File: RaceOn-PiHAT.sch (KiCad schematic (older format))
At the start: 66 parts, among them IC1 MIC29302WU, IC2 NCP5901B, IC3 NCP5901B, IC4 BD48K60G, IC5 LMR14030, J1 BATTERY, J2 ACCELEROMETER, J3 Pi Connector, J4 Encoder Left, J5 Encoder Right, M1 SERVO, M2 MOTOR, Q1 Si7288DP, Q2 Si7288DP, Q3 SQJA37EP1

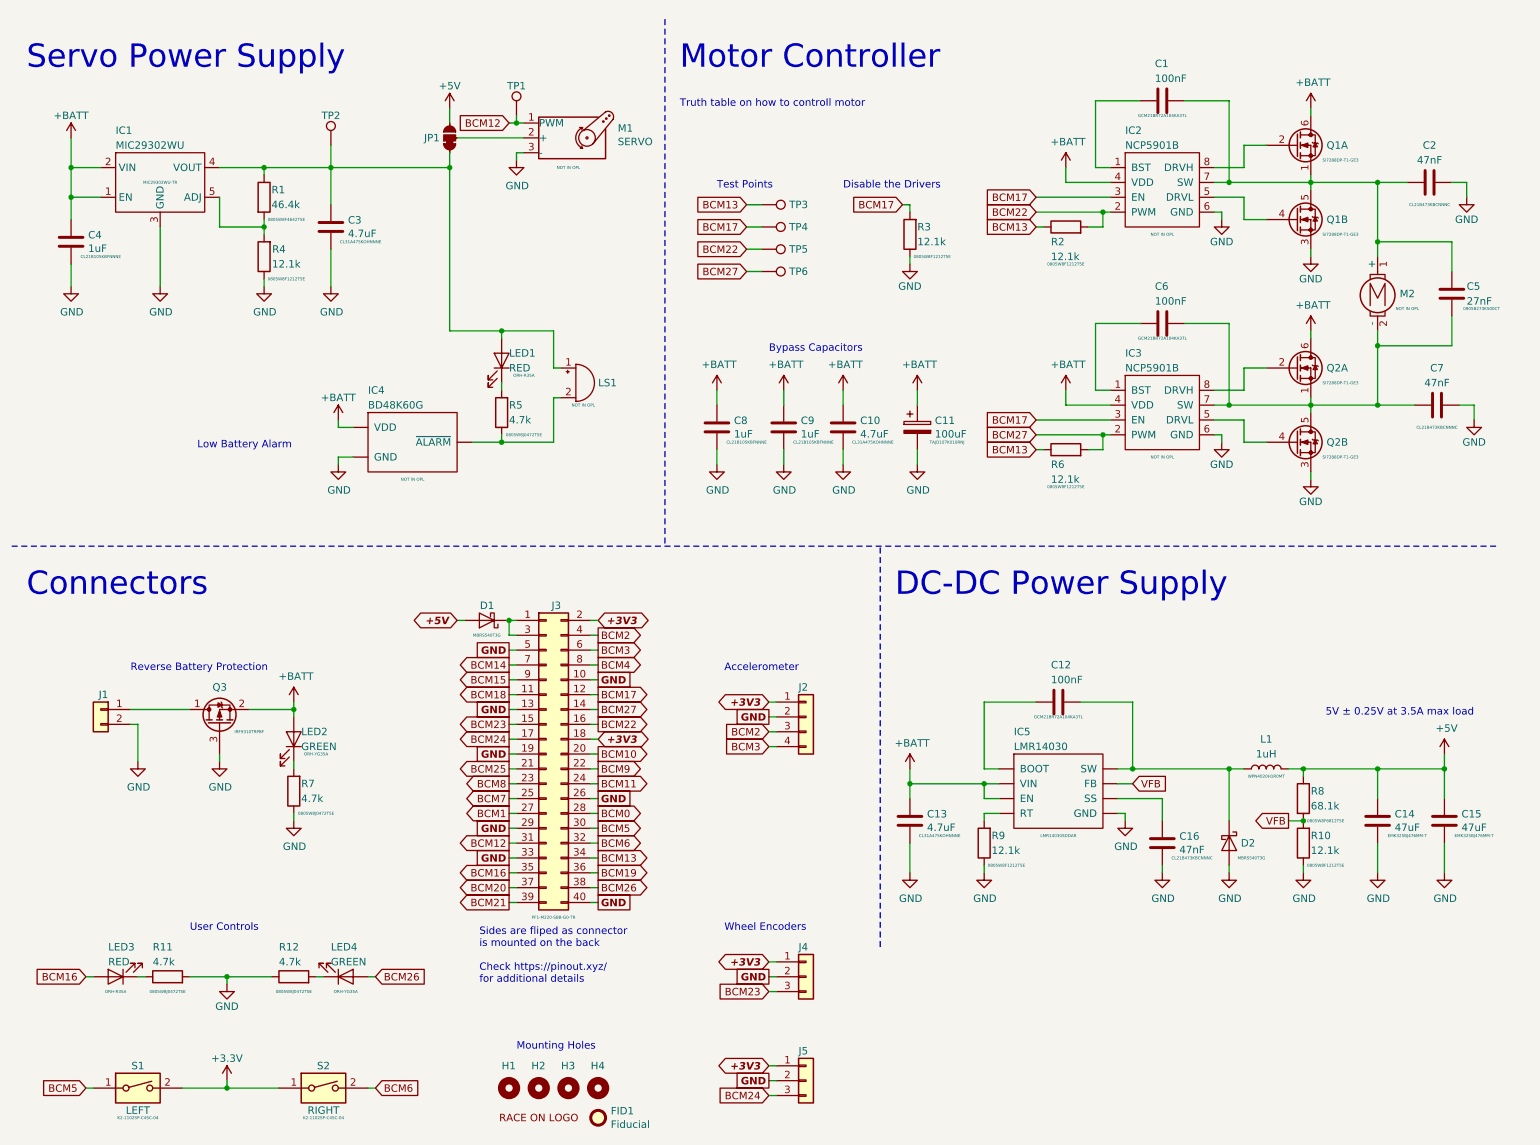
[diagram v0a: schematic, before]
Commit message: Version 2
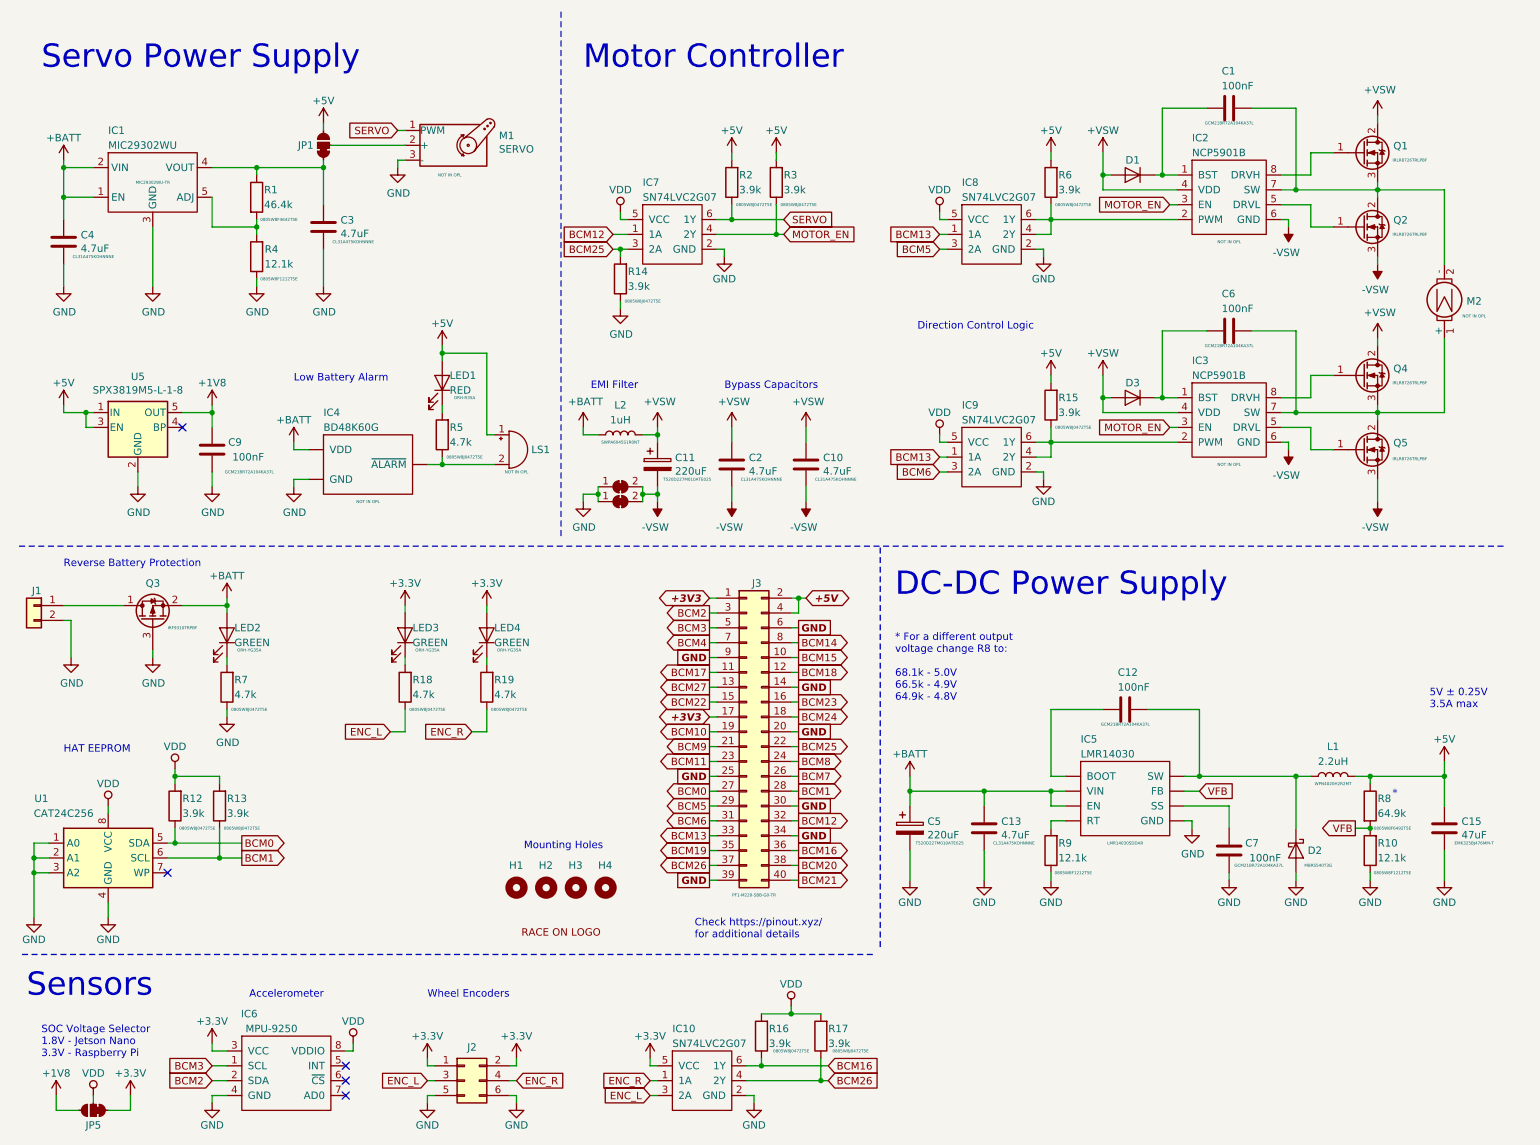
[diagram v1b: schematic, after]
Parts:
- removed C14: 47uF, Race On:CAPC320X250X270L60M, symbol Device:C
- removed C16: 47nF, Race On:CAPC200X125X95L45M, symbol Device:C
- removed C5: 27nF, Race On:CAPC200X125X95L45M, symbol Device:C
- removed C8: 1uF, Race On:CAPC200X125X95L45M, symbol Device:C
- removed D1: D_Schottky, Race On:DIOM795X590X261L117X305M, symbol Device:D_Schottky
- removed FID1: Fiducial, Race On:FID1M3, symbol Mechanical:Fiducial
- removed J2: ACCELEROMETER, Race On:HDRV4W64P254_4X1_1016X254H854, symbol Connector_Generic:Conn_01x04
- removed J4: Encoder Left, Race On:HDRV3W64P254_3X1_762X254H854, symbol Connector_Generic:Conn_01x03
- removed J5: Encoder Right, Race On:HDRV3W64P254_3X1_762X254H854, symbol Connector_Generic:Conn_01x03
- removed Q1, Q2: Si7288DP, Race On:ICSOFL8P127_515X615X112L61X42M, symbol RaceOn-PiHAT:Si7288DP
- removed R11: 4.7k, Race On:RESC200X127X65L40M, symbol Device:R
- removed S1: LEFT, Race On:BTN4P450_600X900X350L83X70M, symbol Switch:SW_DIP_x01
- removed S2: RIGHT, Race On:BTN4P450_600X900X350L83X70M, symbol Switch:SW_DIP_x01
- removed TP1, TP2, TP3, TP4, TP5, TP6: TestPoint, Race On:TESTPOINT, symbol Connector:TestPoint
- added C5: 220uF, Race On:CAPPM730X435X310L135X240L, symbol Device:CP
- added D1, D3: D, Race On:SOD350X160X120L45X62M, symbol Device:D
- added IC10, IC7, IC8, IC9: SN74LVC2G07, Race On:SOT23-6P95_280X145L45X37M, symbol RaceOn-PiHAT:SN74LVC2G07
- added IC6: MPU-9250, Race On:PGA28P254C7R4L1840X1127H200, symbol RaceOn-PiHAT:MPU-9250
- added J2: Conn_02x03_Odd_Even, Race On:HDRV6W65P254_3X2_762X508H900, symbol Connector_Generic:Conn_02x03_Odd_Even
- added JP2, JP3: SolderJumper_2_Bridged, Jumper:SolderJumper-2_P1.3mm_Bridged_Pad1.0x1.5mm, symbol Jumper:SolderJumper_2_Bridged
- added JP5: SolderJumper, Race On:SJ3B12P10X15, symbol RaceOn-PiHAT:SolderJumper
- added L2: 1uH, Race On:INDM600X600X450L155X490M, symbol Device:L
- added Q1, Q2, Q4, Q5: IPD50R380CE, Race On:DPAK3P460_990X239L160X76T650X546L, symbol Transistor_FET:IPD50R380CE
- added R13, R14, R15, R16, R17: 3.9k, Race On:RESC200X127X65L40M, symbol Device:R
- added R18, R19: 4.7k, Race On:RESC200X127X65L40M, symbol Device:R
- added U1: CAT24C256, Race On:SOIC8P127_490X600X175L83X42M, symbol Memory_EEPROM:CAT24C256
- added U5: SPX3819M5-L-1-8, Race On:SOT23-5P95_280X145L45X40M, symbol Regulator_Linear:SPX3819M5-L-1-8
- C11: value 100uF -> 220uF; MPN TAJD107K010RNJ -> T520D227M010ATE025
- C2: value 47nF -> 4.7uF; footprint Race On:CAPC200X125X95L45M -> Race On:CAPC320X160X180L50M; MPN CL21B473KBCNNNC -> CL31A475KOHNNNE
- C4: value 1uF -> 4.7uF; footprint Race On:CAPC200X125X95L45M -> Race On:CAPC320X160X180L50M; MPN CL21B105KBFNNNE -> CL31A475KOHNNNE
- C7: value 47nF -> 100nF; MPN CL21B473KBCNNNC -> GCM21BR72A104KA37L
- C9: value 1uF -> 100nF; MPN CL21B105KBFNNNE -> GCM21BR72A104KA37L
- L1: value 1uH -> 2.2uH; MPN WPN4020H1R0MT -> WPN4020H2R2MT
- LED3: value RED -> GREEN; MPN ORH-R35A -> ORH-YG35A
- R12: value 4.7k -> 3.9k
- R2, R3, R6: value 12.1k -> 3.9k; MPN 0805W8F1212T5E -> 0805W8J0472T5E
- R8: value 68.1k -> 64.9k; MPN 0805W8F6812T5E -> 0805W8F6492T5E
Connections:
- net +3V3: now also J3.1 (Pin_1), J3.17 (Pin_17), LED3.2 (A), LED4.2 (A), IC10.5 (VCC), IC6.3 (VCC), J2.1 (Pin_1), J2.2 (Pin_2), JP5.1 (A); no longer J3.18 (Pin_18), J3.2 (Pin_2)
- net +5V: now also J3.2 (Pin_2), J3.4 (Pin_4), LED1.2 (A), LS1.1 (-), R2.2, R3.2, R6.2, R15.2, U5.1 (IN), U5.3 (EN)
- net +BATT: now also C5.1, L2.2; no longer C10.2, C11.1, C9.2, IC2.4 (VDD), IC3.4 (VDD)
- net BCM0: now also J3.27 (Pin_27), R12.1, U1.5 (SDA); no longer J3.28 (Pin_28)
- net BCM1: now also J3.28 (Pin_28), R13.1, U1.6 (SCL); no longer J3.27 (Pin_27)
- net BCM10: now also J3.19 (Pin_19); no longer J3.20 (Pin_20)
- net BCM11: now also J3.23 (Pin_23); no longer J3.24 (Pin_24)
- net BCM12: now also J3.32 (Pin_32), IC7.1 (1A); no longer J3.31 (Pin_31), M1.1 (PWM)
- net BCM13: now also J3.33 (Pin_33), IC8.1 (1A), IC9.1 (1A); no longer J3.34 (Pin_34), R2.1, R6.1
- net BCM14: now also J3.8 (Pin_8); no longer J3.7 (Pin_7)
- net BCM15: now also J3.10 (Pin_10); no longer J3.9 (Pin_9)
- net BCM16: now also J3.36 (Pin_36), IC10.6 (1Y), R16.1; no longer J3.35 (Pin_35), LED3.2 (A)
- net BCM17: now also J3.11 (Pin_11); no longer IC2.3 (EN), IC3.3 (EN), J3.12 (Pin_12), R3.2
- net BCM18: now also J3.12 (Pin_12); no longer J3.11 (Pin_11)
- net BCM19: now also J3.35 (Pin_35); no longer J3.36 (Pin_36)
- net BCM2: now also J3.3 (Pin_3), IC6.2 (SDA); no longer J3.4 (Pin_4)
- net BCM20: now also J3.38 (Pin_38); no longer J3.37 (Pin_37)
- net BCM21: now also J3.40 (Pin_40); no longer J3.39 (Pin_39)
- net BCM22: now also J3.15 (Pin_15); no longer IC2.2 (PWM), J3.16 (Pin_16), R2.2
- net BCM23: now also J3.16 (Pin_16); no longer J3.15 (Pin_15)
- net BCM24: now also J3.18 (Pin_18); no longer J3.17 (Pin_17)
- net BCM25: now also J3.22 (Pin_22), IC7.3 (2A), R14.2; no longer J3.21 (Pin_21)
- net BCM26: now also J3.37 (Pin_37), IC10.4 (2Y), R17.1; no longer J3.38 (Pin_38), LED4.2 (A)
- net BCM27: now also J3.13 (Pin_13); no longer IC3.2 (PWM), J3.14 (Pin_14), R6.2
- net BCM3: now also J3.5 (Pin_5), IC6.1 (SCL); no longer J3.6 (Pin_6)
- net BCM4: now also J3.7 (Pin_7); no longer J3.8 (Pin_8)
- net BCM5: now also J3.29 (Pin_29), IC8.3 (2A); no longer J3.30 (Pin_30)
- net BCM6: now also J3.31 (Pin_31), IC9.3 (2A); no longer J3.32 (Pin_32)
- net BCM7: now also J3.26 (Pin_26); no longer J3.25 (Pin_25)
- net BCM8: now also J3.24 (Pin_24); no longer J3.23 (Pin_23)
- net BCM9: now also J3.21 (Pin_21); no longer J3.22 (Pin_22)
- net GND: now also J3.14 (Pin_14), J3.20 (Pin_20), J3.25 (Pin_25), J3.30 (Pin_30), J3.34 (Pin_34), J3.39 (Pin_39), J3.6 (Pin_6), J3.9 (Pin_9), C5.2, IC10.2 (GND), IC6.4 (GND), IC7.2 (GND), IC8.2 (GND), IC9.2 (GND), J2.5 (Pin_5), J2.6 (Pin_6), JP2.1 (A), JP3.1 (A), R14.1, U1.1 (A0), U1.2 (A1), U1.3 (A2), U1.4 (GND), U5.2 (GND); no longer C10.1, C11.2, C2.1, IC2.6 (GND), IC3.6 (GND), J3.10 (Pin_10), J3.13 (Pin_13), J3.19 (Pin_19), J3.26 (Pin_26), J3.29 (Pin_29), J3.33 (Pin_33), J3.40 (Pin_40), J3.5 (Pin_5), R12.1, R3.1
- net at C3.2, IC1.4 (VOUT), JP1.1 (A)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: no longer LED1.2 (A), LS1.1 (-)
- net at C6.2, IC3.1 (BST): now also D3.1 (K)
- net at IC3.5 (DRVL): now also Q5.1 (G)
- net at C6.1, IC3.7 (SW): now also M2.1 (+), Q4.3 (S), Q5.2 (D); no longer C7.2, M2.2 (-)
- net at IC3.8 (DRVH): now also Q4.1 (G)
- net at C1.1, IC2.7 (SW): now also M2.2 (-), Q1.3 (S), Q2.2 (D); no longer C2.2, M2.1 (+)
- net at C1.2, IC2.1 (BST): now also D1.1 (K)
- net at IC2.5 (DRVL): now also Q2.1 (G)
- net at IC2.8 (DRVH): now also Q1.1 (G)
- net at LED3.1 (K): now also R18.2
- net at LED4.1 (K): now also R19.2; no longer R12.2
- net at IC5.6 (SS): now also C7.2
- new net: IC3.2 (PWM), IC9.4 (2Y), IC9.6 (1Y), R15.1
- new net: IC2.2 (PWM), IC8.4 (2Y), IC8.6 (1Y), R6.1
- new net +1V8: C9.2, JP5.3 (B), U5.5 (OUT)
- new net +VSW: C10.2, C11.1, C2.2, D1.2 (A), D3.2 (A), IC2.4 (VDD), IC3.4 (VDD), L2.1, Q1.2 (D), Q4.2 (D)
- new net -VSW: C10.1, C11.2, C2.1, IC2.6 (GND), IC3.6 (GND), JP2.2 (B), JP3.2 (B), Q2.3 (S), Q5.3 (S)
- new net ENC_L: IC10.3 (2A), J2.3 (Pin_3), R18.1
- new net ENC_R: IC10.1 (1A), J2.4 (Pin_4), R19.1
- new net MOTOR_EN: IC2.3 (EN), IC3.3 (EN), IC7.4 (2Y), R3.1
- new net SERVO: IC7.6 (1Y), M1.1 (PWM), R2.1
- new net VDD: IC6.8 (VDDIO), IC7.5 (VCC), IC8.5 (VCC), IC9.5 (VCC), JP5.2 (C), R12.2, R13.2, R16.2, R17.2, U1.8 (VCC)
- no-connect marks 0 -> 5
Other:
- note added: "*"
- note added: "* For a different output \nvoltage change R8 to:\n\n68.1k - 5.0V\n66.5k - 4.9V\n64.9k - 4.8V"
- note added: "5V ± 0.25V\n3.5A max"
- note added: "Check https://pinout.xyz/\nfor additional details\n"
- note added: "Direction Control Logic"
- note added: "EMI Filter"
- note added: "HAT EEPROM"
- note added: "SOC Voltage Selector\n1.8V - Jetson Nano\n3.3V - Raspberry Pi"
- note added: "Sensors\n"
- note removed: "5V ± 0.25V at 3.5A max load"
- note removed: "Connectors"
- note removed: "Disable the Drivers"
- note removed: "Sides are fliped as connector\nis mounted on the back\n\nCheck https://pinout.xyz/\nfor additional details\n"
- note removed: "Test Points"
- note removed: "Truth table on how to controll motor"
- note removed: "User Controls"
- moved on the sheet: C1, C10, C11, C12, C13, C15, C3, C6, D2, H1, H2, H3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
